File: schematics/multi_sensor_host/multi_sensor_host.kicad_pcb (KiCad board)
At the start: 2 copper layers, 169 parts, among them J1 left hand 0, J10 swd, J11 stm_boot, J13 right hand 0, J14 right hand 1, J15 right hand 2, J16 right hand 3, J17 rst_mcu, J18 left hand 3, J19 left leg 0, J2 left hand 1, J20 left leg 1, J21 right lef 0, J22 right leg 1, J3 bm_cfg, J4 left hand 2, J5 tx, J6 MY_USB_B, J7 rst_bm71, J8 rx, J9 uart1, U1 TCA9548A_TSSOP, U11 MCP111, U12 BM71BLES1FC2-0B02AA, U2 TCA9548A_TSSOP, U3 TCA9548A_TSSOP, U4 MCP111, U5 TPS79333-EP, U8 MCP73812, U9 MCP1603, Y1 Crystal

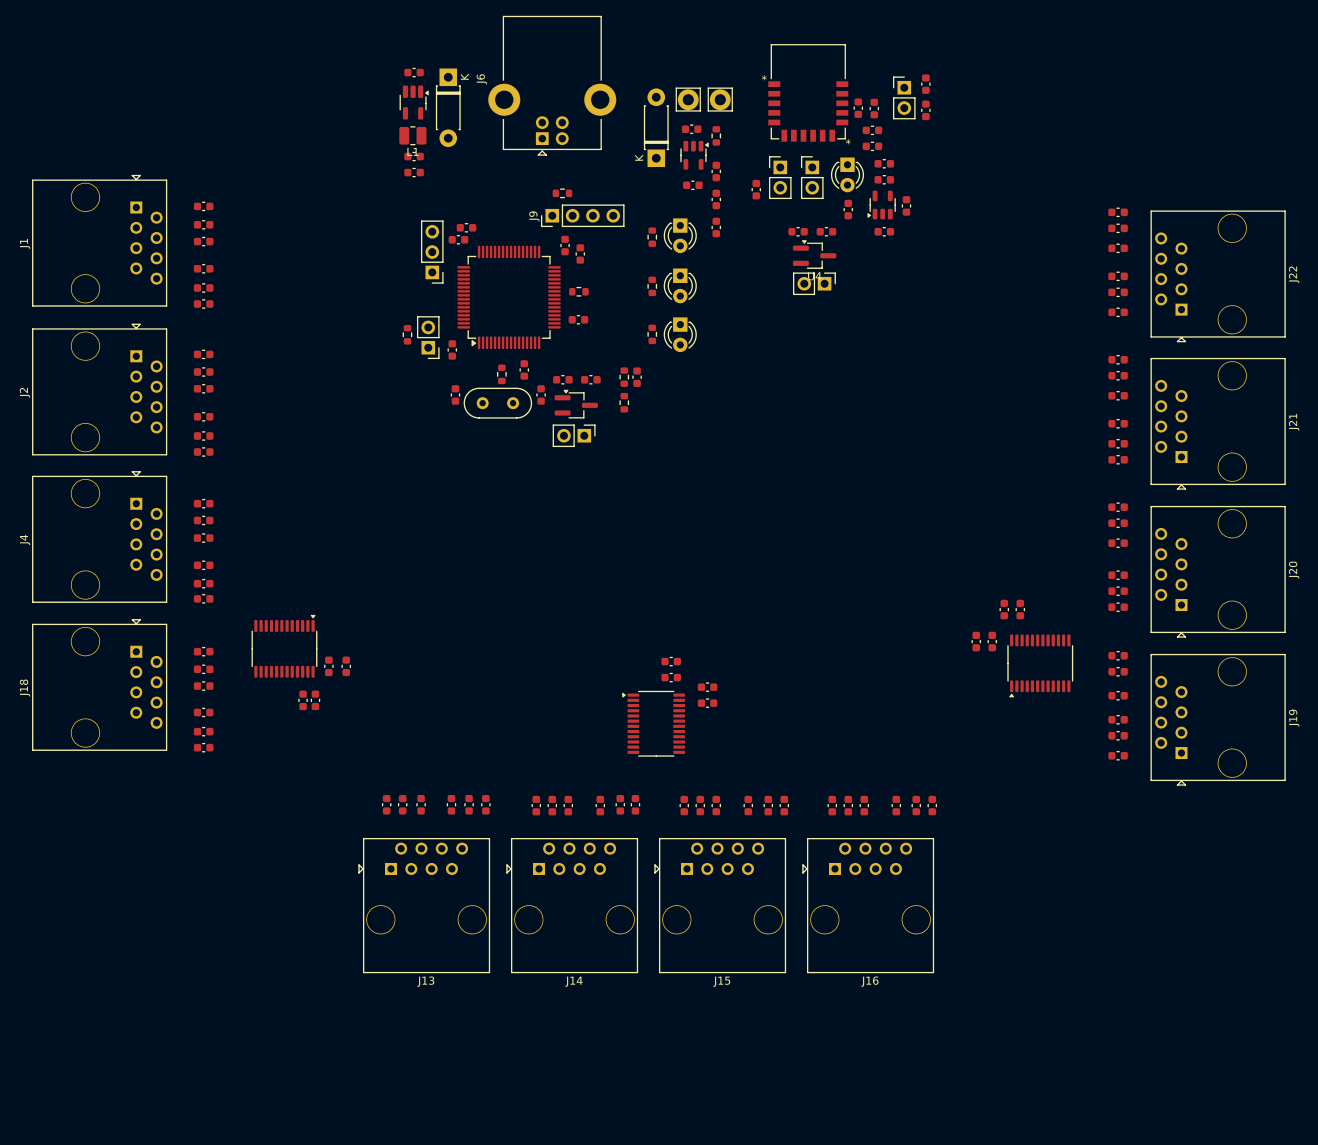
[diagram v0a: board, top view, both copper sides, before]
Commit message: a
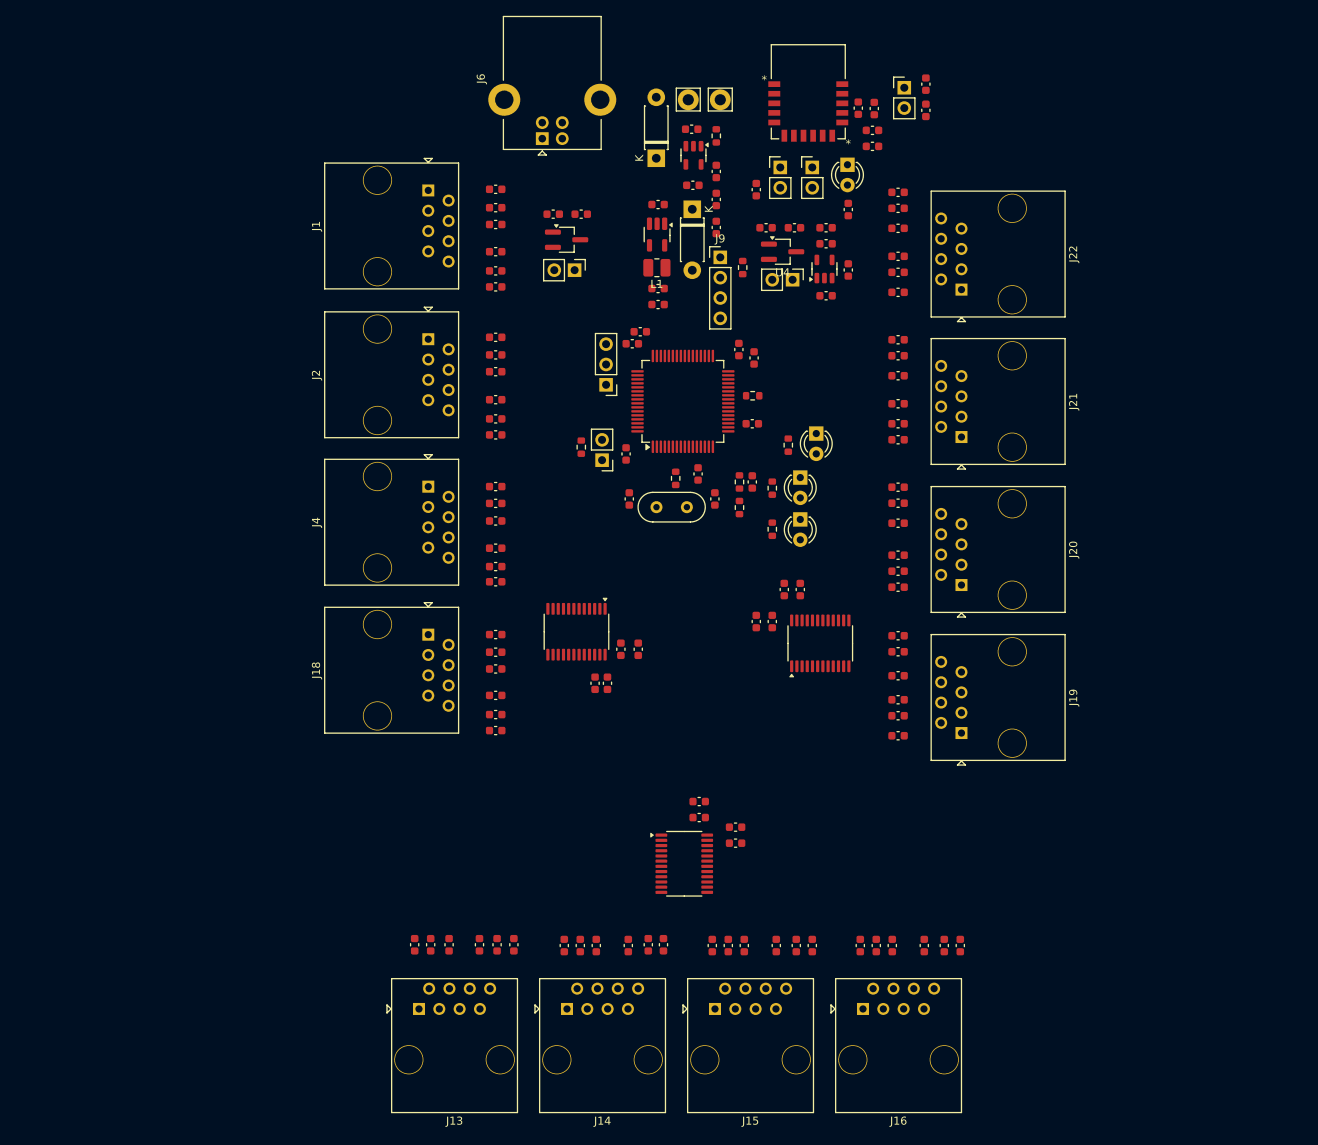
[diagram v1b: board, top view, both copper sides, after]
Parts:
- moved C40 36.6 mm to (84.9, 131.4)
- moved C41 36.6 mm to (84.9, 129.4)
- moved R2 36.6 mm to (98.9, 125.4)
- moved U1 36.6 mm to (95.0, 119.0)
- moved C1 36.6 mm to (100.6, 121.2)
- moved C19 36.6 mm to (84.9, 94.4)
- moved C2 36.6 mm to (102.7, 121.2)
- moved C20 36.6 mm to (84.9, 92.4)
- moved C36 36.6 mm to (84.9, 75.9)
- moved C37 36.6 mm to (84.9, 73.9)
- moved C44 36.6 mm to (84.9, 112.8)
- moved C45 36.6 mm to (84.9, 110.9)
- moved J1 36.6 mm to (76.5, 63.8)
- moved J18 36.6 mm to (76.5, 119.4)
- moved J2 36.6 mm to (76.5, 82.4)
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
